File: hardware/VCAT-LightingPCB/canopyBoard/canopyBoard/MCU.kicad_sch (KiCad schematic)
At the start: 6 parts

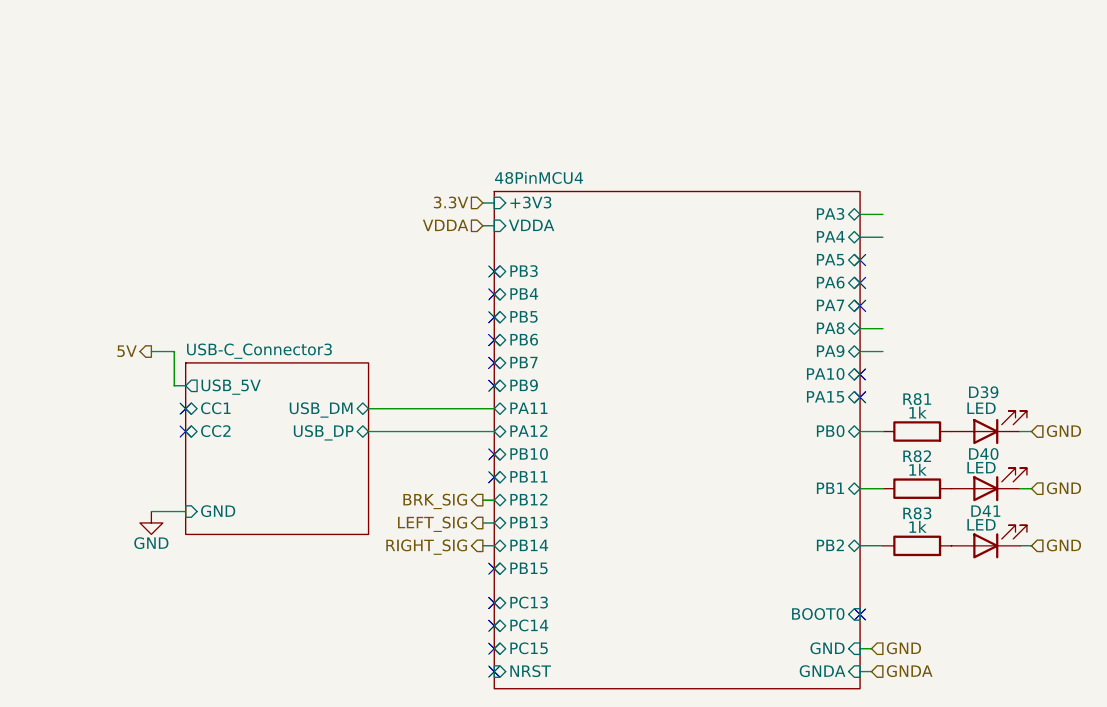
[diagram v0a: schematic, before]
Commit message: added current check, please dont overwrite my file again
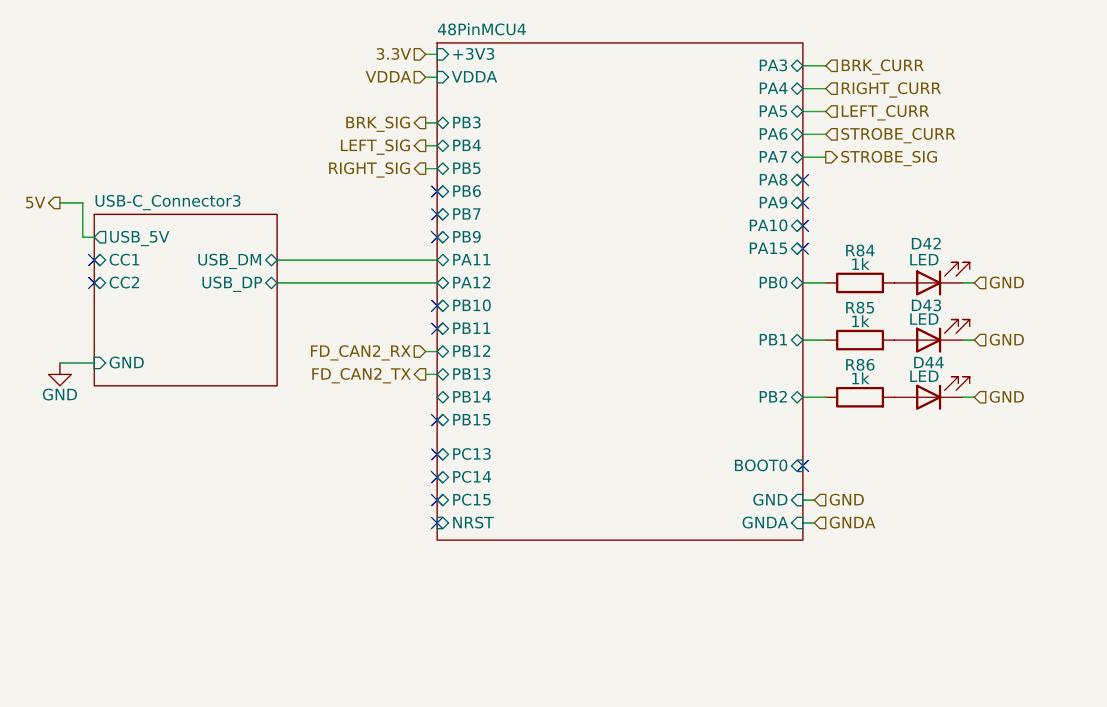
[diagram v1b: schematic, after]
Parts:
- removed D39, D40, D41: LED, symbol Device:LED
- removed R81, R82, R83: 1k, symbol Device:R
- added D42, D43, D44: LED, symbol Device:LED
- added R84, R85, R86: 1k, symbol Device:R
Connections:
- net 48PinMCU4/PB0: now also R84.1
- net 48PinMCU4/PB1: now also R85.1
- net 48PinMCU4/PB2: now also R86.1
- net GND: now also D42.1 (K), D43.1 (K), D44.1 (K)
- new net: D42.2 (A), R84.2
- new net: D44.2 (A), R86.2
- new net: D43.2 (A), R85.2
- no-connect marks 21 -> 17
